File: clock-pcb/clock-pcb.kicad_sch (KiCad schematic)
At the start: 61 parts, among them J1 Conn_01x03_Pin, J10 Conn_01x01_Socket, J11 Conn_01x01_Socket, J12 Conn_01x01_Socket, J13 Conn_01x01_Socket, J14 Conn_01x01_Socket, J15 Conn_01x02_Socket, J2 oled, J3 Led display, J4 Led display 2, J5 Conn_01x07_Socket, J6 Conn_01x07_Socket, J7 Conn_01x01_Socket, J8 Conn_01x02_Socket, J9 Conn_01x01_Socket, Q1 FS8205A, Q2 FDN304PZ, U1 ESP32-WROOM-E, U4 TPS2116DRL, U5 MCP73811T-420I-OT, U7 TLV75533PDBV

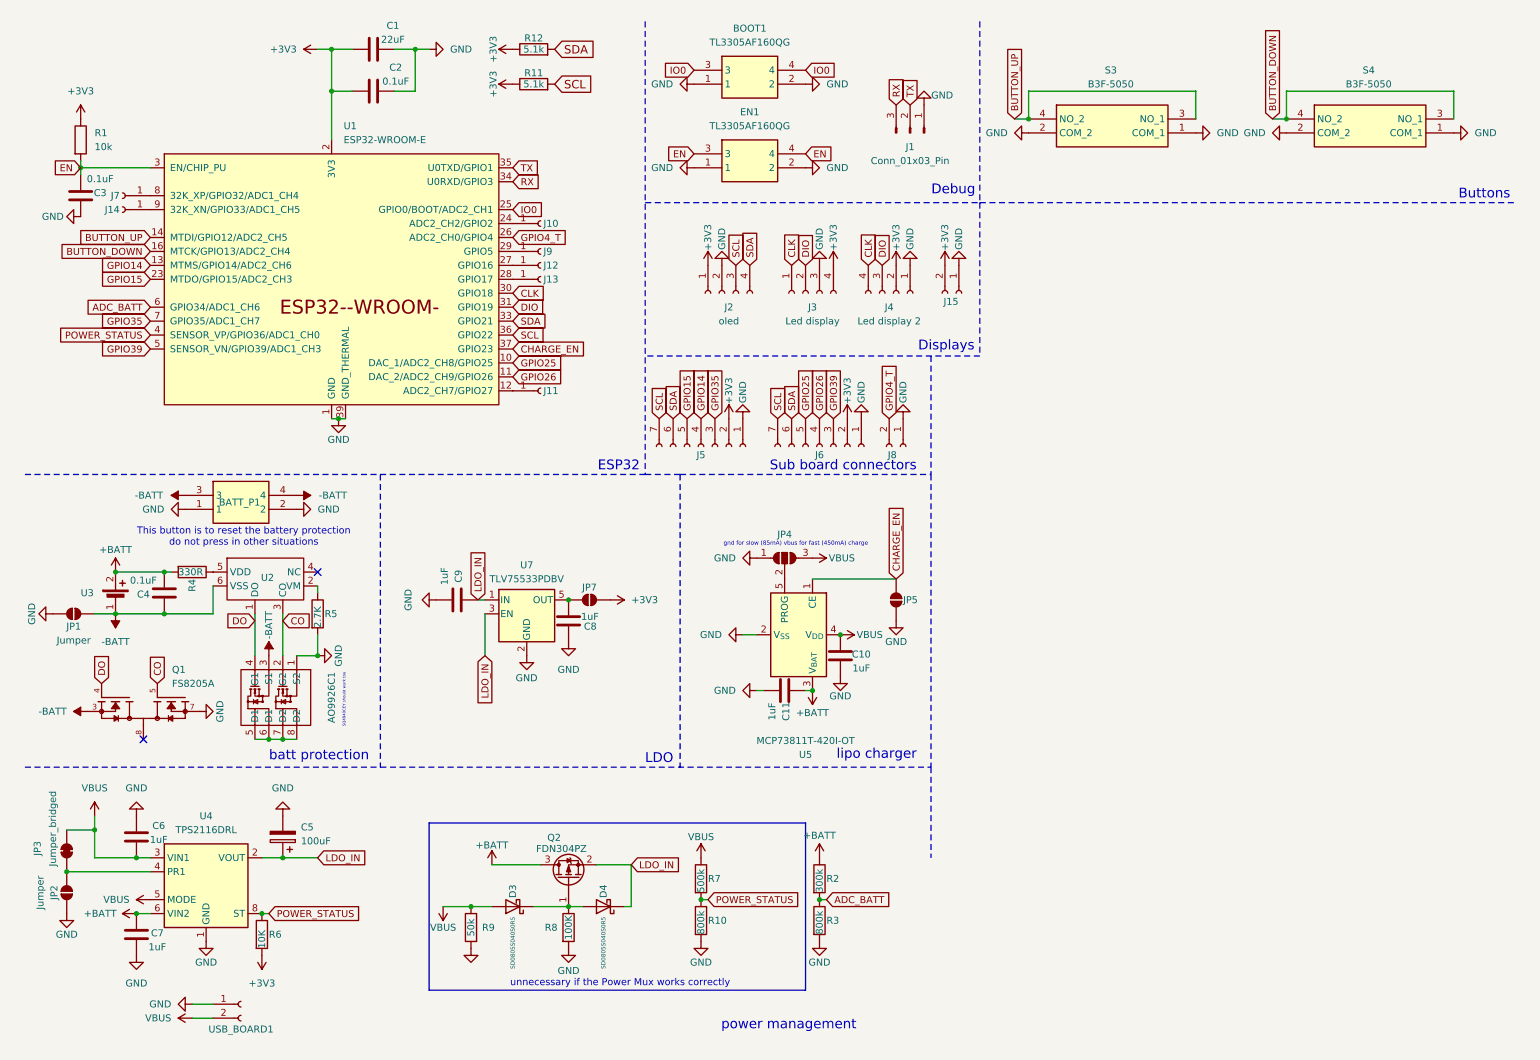
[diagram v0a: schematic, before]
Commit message: new pcb
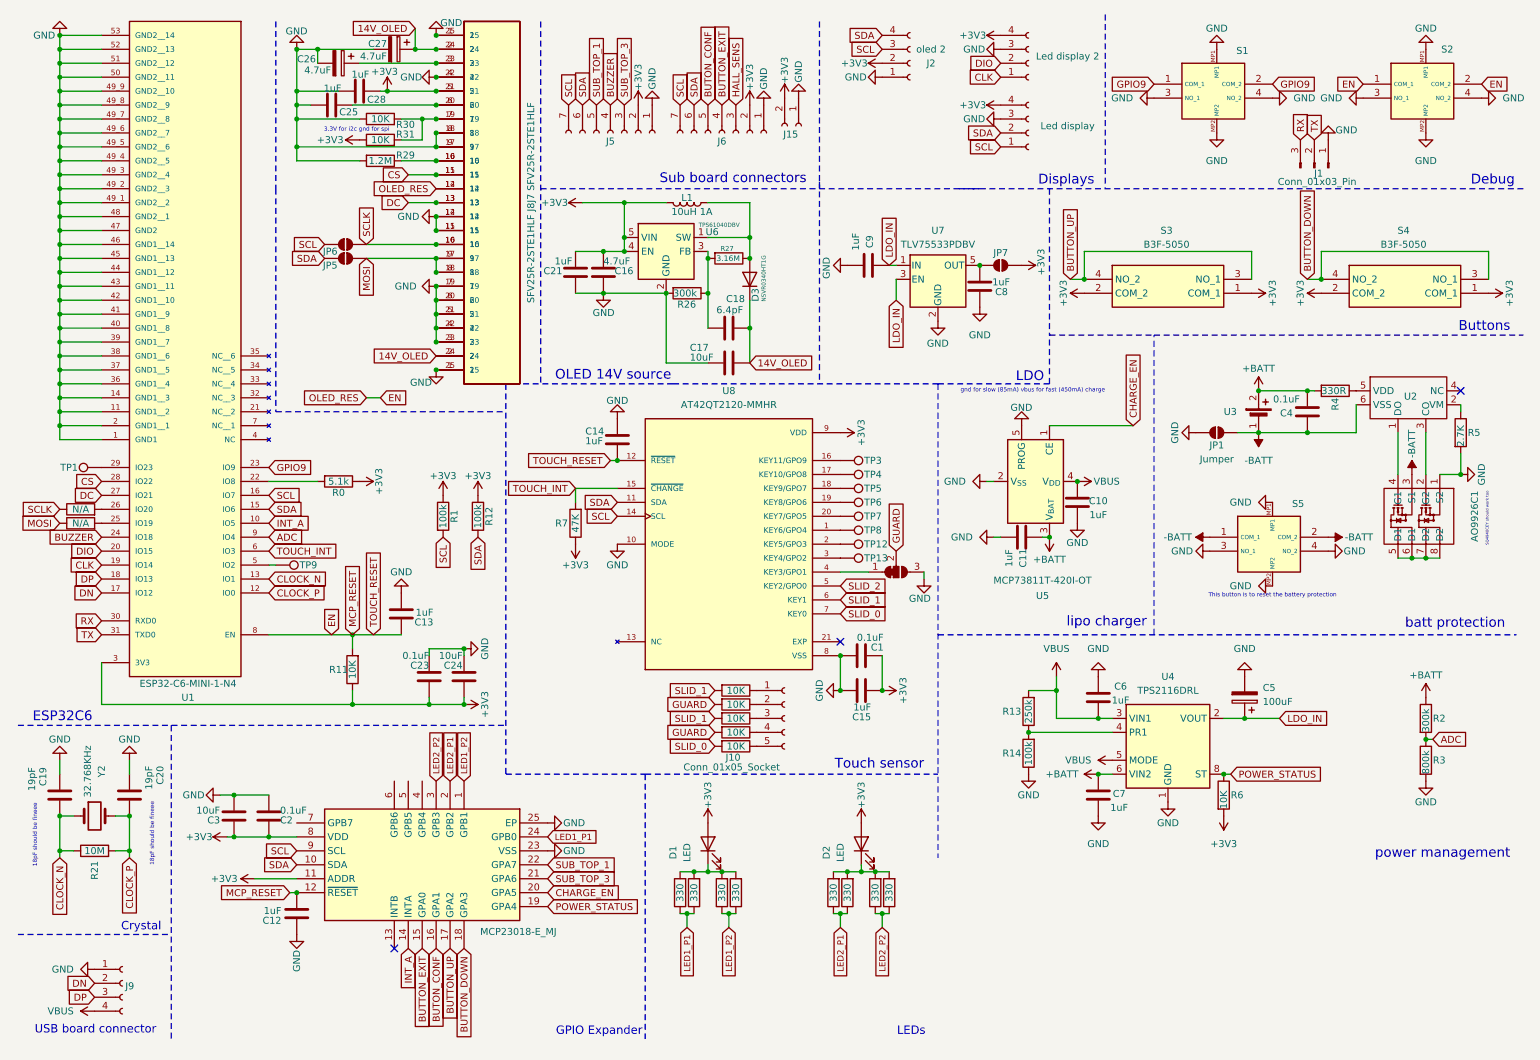
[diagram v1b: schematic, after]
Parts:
- removed BATT_P1, BOOT1, EN1: TL3305AF160QG, clock:TL3305AF160QG, symbol clock:TL3305AF160QG
- removed C1: 22uF, Capacitor_SMD:C_0805_2012Metric, symbol clock:C
- removed C2, C3: 0.1uF, Capacitor_SMD:C_0603_1608Metric, symbol clock:C
- removed D3, D4: SD0805S040S0R5, Diode_SMD:D_0805_2012Metric, symbol Watchy:D_Schottky
- removed J10, J11, J12, J13, J14, J7, J9: Conn_01x01_Socket, Connector_PinSocket_2.54mm:PinSocket_1x01_P2.54mm_Vertical, symbol Connector:Conn_01x01_Socket
- removed J5, J6: Conn_01x07_Socket, Connector_PinSocket_2.54mm:PinSocket_1x07_P2.54mm_Vertical, symbol Connector:Conn_01x07_Socket
- removed J8: Conn_01x02_Socket, Connector_PinSocket_2.54mm:PinSocket_1x02_P2.54mm_Vertical, symbol Connector:Conn_01x02_Socket
- removed JP2: Jumper, Jumper:SolderJumper-2_P1.3mm_Open_RoundedPad1.0x1.5mm, symbol Jumper:SolderJumper_2_Open
- removed JP3: Jumper_bridged, Jumper:SolderJumper-2_P1.3mm_Bridged2Bar_RoundedPad1.0x1.5mm, symbol Jumper:SolderJumper_2_Bridged
- removed JP4: SolderJumper_3_Open, Jumper:SolderJumper-3_P1.3mm_Open_RoundedPad1.0x1.5mm, symbol Jumper:SolderJumper_3_Open
- removed Q1: FS8205A, clock:SOP65P640X120-8N, symbol FS8205A:FS8205A
- removed Q2: FDN304PZ, Package_TO_SOT_SMD:SOT-23, symbol Watchy:BSS83P
- removed R1: 10k, Resistor_SMD:R_0402_1005Metric, symbol clock:R
- removed R10: 800k, Resistor_SMD:R_0402_1005Metric, symbol clock:R
- removed R7: 500k, Resistor_SMD:R_0402_1005Metric, symbol clock:R
- removed U1: ESP32-WROOM-E, PCM_Espressif:ESP32-WROOM-32E, symbol clock:ESP32-WROOM-E
- removed USB_BOARD1: Conn_01x02_Socket, clock:SHDR2W64P0X250_1X2_740X575X700P, symbol clock:Conn_01x02_Socket
- added C1, C2, C23: 0.1uF, Capacitor_SMD:C_0603_1608Metric, symbol Watchy:C
- added C12, C13, C14, C15, C21, C25, C28: 1uF, Capacitor_SMD:C_0603_1608Metric, symbol Watchy:C
- added C16: 4.7uF, Capacitor_SMD:C_0805_2012Metric, symbol Watchy:C
- added C17, C24, C3: 10uF, Capacitor_SMD:C_0603_1608Metric, symbol Watchy:C
- added C18: 6.4pF, Capacitor_SMD:C_0402_1005Metric, symbol Watchy:C
- added C19, C20: 19pF, Capacitor_SMD:C_0402_1005Metric, symbol Watchy:C
- added C26, C27: 4.7uF, Capacitor_Tantalum_SMD:CP_EIA-3528-12_Kemet-T, symbol Device:C_Polarized
- added D1, D2: LED, LED_SMD:LED_1210_3225Metric, symbol Device:LED
- added D3: NSVR0340HT1G, Diode_SMD:D_SOD-323, symbol Device:D
- added IC2: MCP23018-E_MJ, clock:QFN50P400X400X90-25N-D, symbol Watchy:MCP23018-E_MJ
- added J10: Conn_01x05_Socket, Connector_PinHeader_2.54mm:PinHeader_1x05_P2.54mm_Vertical, symbol Connector:Conn_01x05_Socket
- added J5, J6: Conn_01x07_Socket, Connector_PinHeader_2.54mm:PinHeader_1x07_P2.54mm_Vertical, symbol clock:Conn_01x07_Socket
- added J7: SFV25R-2STE1HLF, clock:OLED_1.5IN_128X128MONO, symbol SFV25R-2STE1HLF:SFV25R-2STE1HLF
- added J8: SFV25R-2STE1HLF, clock:AMPHENOL_SFV25R-2STE1HLF, symbol SFV25R-2STE1HLF:SFV25R-2STE1HLF
- added J9: Conn_01x04_Socket, Connector_JST:JST_XH_B4B-XH-AM_1x04_P2.50mm_Vertical, symbol Connector:Conn_01x04_Socket
- added JP2: SolderJumper_3_Bridged12, clock:jumper_solder_small_3_bridged, symbol Jumper:SolderJumper_3_Bridged12
- added JP6: Jumper, clock:jumper_solder_small, symbol Jumper:SolderJumper_2_Open
- added L1: 10uH 1A, clock:HPI0530-100, symbol Watchy:L
- added R0: 5.1k, Resistor_SMD:R_0402_1005Metric, symbol Watchy:R
- added R1, R14: 100k, Resistor_SMD:R_0402_1005Metric, symbol Watchy:R
- added R10, R15, R16, R30, R31: 10K, Resistor_SMD:R_0402_1005Metric, symbol Watchy:R
- added R13: 250k, Resistor_SMD:R_0402_1005Metric, symbol Watchy:R
- added R17, R18, R19, R20, R22, R23, R24, R25: 330, Resistor_SMD:R_0402_1005Metric, symbol Yatchy:R
- added R21: 10M, Resistor_SMD:R_0402_1005Metric, symbol Watchy:R
- added R26: 300k, Resistor_SMD:R_0402_1005Metric, symbol Watchy:R
- added R27: 3.16M, Resistor_SMD:R_0402_1005Metric, symbol Watchy:R
- added R29: 1.2M, Resistor_SMD:R_0402_1005Metric, symbol Watchy:R
- added R32, R33: N/A, Resistor_SMD:R_0402_1005Metric, symbol Watchy:R
- added R7: 47K, Resistor_SMD:R_0402_1005Metric, symbol Watchy:R
- added S1, S2, S5: TS21-34-035-BK-160-SMT-TR, TS2134035BK160SMTTR, symbol TS21-34-035-BK-160-SMT-TR:TS21-34-035-BK-160-SMT-TR
- added TP1, TP12, TP13, TP3, TP4, TP5, TP6, TP7, TP8, TP9: TestPoint, TestPoint:TestPoint_THTPad_1.0x1.0mm_Drill0.5mm, symbol Connector:TestPoint
- added U1: ESP32-C6-MINI-1-N4, clock:XCVR_ESP32-C6-MINI-1-N4, symbol Watchy:ESP32-C6-MINI-1-N4
- added U6: TPS61040DBV, Package_TO_SOT_SMD:SOT-23-5, symbol Regulator_Switching:TPS61040DBV
- added U8: AT42QT2120-MMHR, clock:QFN45P300X300X85-21N, symbol AT42QT2120-MMHR:AT42QT2120-MMHR
- added Y2: 32.768KHz, clock:XTAL_9HT10_TXC, symbol Watchy:Crystal
- J2: value oled -> oled 2
- JP1, JP7: footprint Jumper:SolderJumper-2_P1.3mm_Open_RoundedPad1.0x1.5mm -> clock:jumper_solder_small
- JP5: value SolderJumper_2_Open -> Jumper; footprint Jumper:SolderJumper-2_P1.3mm_Open_RoundedPad1.0x1.5mm -> clock:jumper_solder_small
- R11: value 5.1k -> 10K
- R12: value 5.1k -> 100k
- R8: value 100K -> 10K
- R9: value 50k -> 10K
- U3: footprint clock:SHDR2W64P0X250_1X2_740X575X700P -> Connector_JST:JST_XH_B2B-XH-AM_1x02_P2.50mm_Vertical
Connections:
- net +3V3: now also J2.2 (Pin_2), J4.4 (Pin_4), S3.1 (COM_1), S3.2 (COM_2), S4.1 (COM_1), S4.2 (COM_2), C1.2, C15.2, C16.1, C2.1, C21.2, C23.1, C24.1, C28.2, C3.1, D1.2 (A), D2.2 (A), IC2.11 (ADDR), IC2.8 (VDD), J5.2 (Pin_2), J6.2 (Pin_2), J7.5, J8.21, L1.2, R0.1, R1.1, R31.1, R7.1, U1.3 (3V3), U6.4 (EN), U6.5 (VIN), U8.9 (VDD); no longer J2.1 (Pin_1), J4.2 (Pin_2)
- net -BATT: now also S5.1 (COM_1), S5.2 (COM_2)
- net BUTTON_DOWN: now also IC2.18 (GPA3)
- net BUTTON_UP: now also IC2.17 (GPA2)
- net CHARGE_EN: now also IC2.20 (GPA5); no longer JP5.2 (B)
- net CLK: now also J4.1 (Pin_1), U1.19 (IO14); no longer J3.1 (Pin_1), J4.4 (Pin_4)
- net DIO: now also J4.2 (Pin_2), U1.20 (IO15); no longer J3.2 (Pin_2), J4.3 (Pin_3)
- net EN: now also R11.2, C12.2, C13.1, C14.2, IC2.12 (~{RESET}), J7.12, J8.14, S2.1 (COM_1), S2.2 (COM_2), U1.8 (EN), U8.12 (~{RESET})
- net GND: now also J2.1 (Pin_1), J4.3 (Pin_3), U5.5 (PROG), C1.1, C12.1, C13.2, C14.1, C15.1, C16.2, C17.2, C19.2, C2.2, C20.2, C21.1, C23.2, C24.2, C25.1, C26.2, C27.2, C28.1, C3.2, IC2.23 (VSS), IC2.25 (EP), J5.1 (Pin_1), J6.1 (Pin_1), J7.1, J7.14, J7.15, J7.19, J7.20, J7.21, J7.22, J7.23, J7.25, J7.4, J7.8, J7.9, J8.1, J8.11, J8.12, J8.17, J8.18, J8.22, J8.25, J8.3, J8.4, J8.5, J8.6, J8.7, J9.1 (Pin_1), JP2.3 (B), R14.1, R26.2, R29.2, R30.1, S1.3 (NO_1), S1.4 (NO_2), S1.MP1, S1.MP2, S2.3 (NO_1), S2.4 (NO_2), S2.MP1, S2.MP2, S5.3 (NO_1), S5.4 (NO_2), S5.MP1, S5.MP2, U1.1 (GND1), U1.11 (GND1__2), U1.14 (GND1__3), U1.2 (GND1__1), U1.36 (GND1__4), U1.37 (GND1__5), U1.38 (GND1__6), U1.39 (GND1__7), U1.40 (GND1__8), U1.41 (GND1__9), U1.42 (GND1__10), U1.43 (GND1__11), U1.44 (GND1__12), U1.45 (GND1__13), U1.46 (GND1__14), U1.47 (GND2), U1.48 (GND2__1), U1.49_1 (GND2__2), U1.49_2 (GND2__3), U1.49_3 (GND2__4), U1.49_4 (GND2__5), U1.49_5 (GND2__6), U1.49_6 (GND2__7), U1.49_7 (GND2__8), U1.49_8 (GND2__9), U1.49_9 (GND2__10), U1.50 (GND2__11), U1.51 (GND2__12), U1.52 (GND2__13), U1.53 (GND2__14), U6.2 (GND), U8.10 (MODE), U8.8 (VSS); no longer J2.2 (Pin_2), J4.1 (Pin_1), JP5.1 (A), R8.2, R9.2, S3.1 (COM_1), S3.2 (COM_2), S4.1 (COM_1), S4.2 (COM_2)
- net POWER_STATUS: now also IC2.19 (GPA4)
- net RX: now also U1.30 (RXD0)
- net SCL: now also J3.1 (Pin_1), IC2.9 (SCL), J5.7 (Pin_7), J6.7 (Pin_7), JP6.1 (A), R1.2, U1.16 (IO7), U8.14 (SCL); no longer R11.2
- net SDA: now also J3.2 (Pin_2), JP5.1 (A), IC2.10 (SDA), J5.6 (Pin_6), J6.6 (Pin_6), U1.15 (IO6), U8.11 (SDA)
- net TX: now also U1.31 (TXD0)
- net VBUS: now also J9.4 (Pin_4), R13.2; no longer R9.1
- net at R8.1: now also J10.5 (Pin_5)
- net at U4.4 (PR1): now also R13.1, R14.2
- net ADC_BATT renamed ADC
- net ADC: now also U1.9 (IO4)
- net CO: no longer names the net of AO9926C1.2 (G2), U2.3 (CO)
- net DO: no longer names the net of AO9926C1.4 (G1), U2.1 (DO)
- new net: D3.2 (A), L1.1, R27.1, U6.1 (SW)
- new net: C18.2, R26.1, R27.2, U6.3 (FB)
- new net: D2.1 (K), R22.2, R23.2, R24.2, R25.2
- new net: J10.2 (Pin_2), R15.1
- new net: TP3.1, U8.16 (KEY11/GPO9)
- new net: D1.1 (K), R17.2, R18.2, R19.2, R20.2
- new net: C26.1, J7.3, J8.23
- new net: TP8.1, U8.1 (KEY6/GPO4)
- new net: TP4.1, U8.17 (KEY10/GPO8)
- new net: TP5.1, U8.18 (KEY9/GPO7)
- new net: TP6.1, U8.19 (KEY8/GPO6)
- new net: TP12.1, U8.2 (KEY5/GPO3)
- new net: TP7.1, U8.20 (KEY7/GPO5)
- new net: TP13.1, U8.3 (KEY4/GPO2)
- new net: JP2.1 (A), U8.4 (KEY3/GPO1)
- new net: J10.4 (Pin_4), R9.1
- new net: R0.2, U1.22 (IO8)
- new net: TP1.1, U1.29 (IO23)
- new net: J10.3 (Pin_3), R10.1
- new net: TP9.1, U1.5 (IO2)
- new net: J7.10, J8.16, R29.1
- new net: C25.2, J7.6, J8.20
- new net: J7.7, J8.19, R30.2, R31.2
- new net: J10.1 (Pin_1), R16.1
- new net: R33.2, U1.25 (IO19)
- new net: R32.2, U1.26 (IO20)
- new net 14V_OLED: C17.1, C18.1, C27.1, D3.1 (K), J7.2, J7.24, J8.2, J8.24
- new net BUTON_CONF: IC2.16 (GPA1), J6.5 (Pin_5)
- new net BUTTON_EXIT: IC2.15 (GPA0), J6.4 (Pin_4)
- new net BUZZER: J5.4 (Pin_4), U1.24 (IO18)
- new net CLOCK_N: C19.1, R21.1, U1.13 (IO1), Y2.1
- new net CLOCK_P: C20.1, R21.2, U1.12 (IO0), Y2.2
- new net CS: J7.11, J8.15, U1.28 (IO22)
- new net DC: J7.13, J8.13, U1.27 (IO21)
- new net DN: J9.2 (Pin_2), U1.17 (IO12)
- new net DP: J9.3 (Pin_3), U1.18 (IO13)
- new net GPIO9: S1.1 (COM_1), S1.2 (COM_2), U1.23 (IO9)
- new net GUARD: JP2.2 (C), R15.2, R9.2
- new net HALL_SENS: J6.3 (Pin_3)
- new net INT_A: IC2.14 (INTA), U1.10 (IO5)
- new net LED1_P1: IC2.24 (GPB0), R17.1, R19.1
- new net LED1_P2: IC2.1 (GPB1), R18.1, R20.1
- new net LED2_P1: IC2.2 (GPB2), R22.1, R23.1
- new net LED2_P2: IC2.3 (GPB3), R24.1, R25.1
- new net MOSI: J7.17, J7.18, J8.8, J8.9, JP5.2 (B), R33.1
- new net SCLK: J7.16, J8.10, JP6.2 (B), R32.1
- new net SLID_0: R8.2, U8.7 (KEY0)
- new net SLID_1: R10.2, R16.2, U8.6 (KEY1)
- new net SLID_2: U8.5 (KEY2/GPO0)
- new net SUB_TOP_1: IC2.22 (GPA7), J5.5 (Pin_5)
- new net SUB_TOP_3: IC2.21 (GPA6), J5.3 (Pin_3)
- new net TOUCH_INT: R7.2, U1.6 (IO3), U8.15 (~{CHANGE})
- no-connect marks 2 -> 3
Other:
- note added: "18pF should be fineee"
- note added: "3.3V for i2c gnd for spi"
- note added: "Crystal"
- note added: "ESP32C6"
- note added: "GPIO Expander"
- note added: "LEDs"
- note added: "OLED 14V source"
- note added: "This button is to reset the battery protection"
- note added: "Touch sensor"
- note added: "USB board connector"
- note removed: "ESP32"
- note removed: "This button is to reset the battery protection do not press in other situations"
- note removed: "unnecessary if the Power Mux works correctly"
- moved on the sheet: AO9926C1, C10, C11, C4, C5, C6, C7, C8, C9, J1, J15, J2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

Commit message: routing
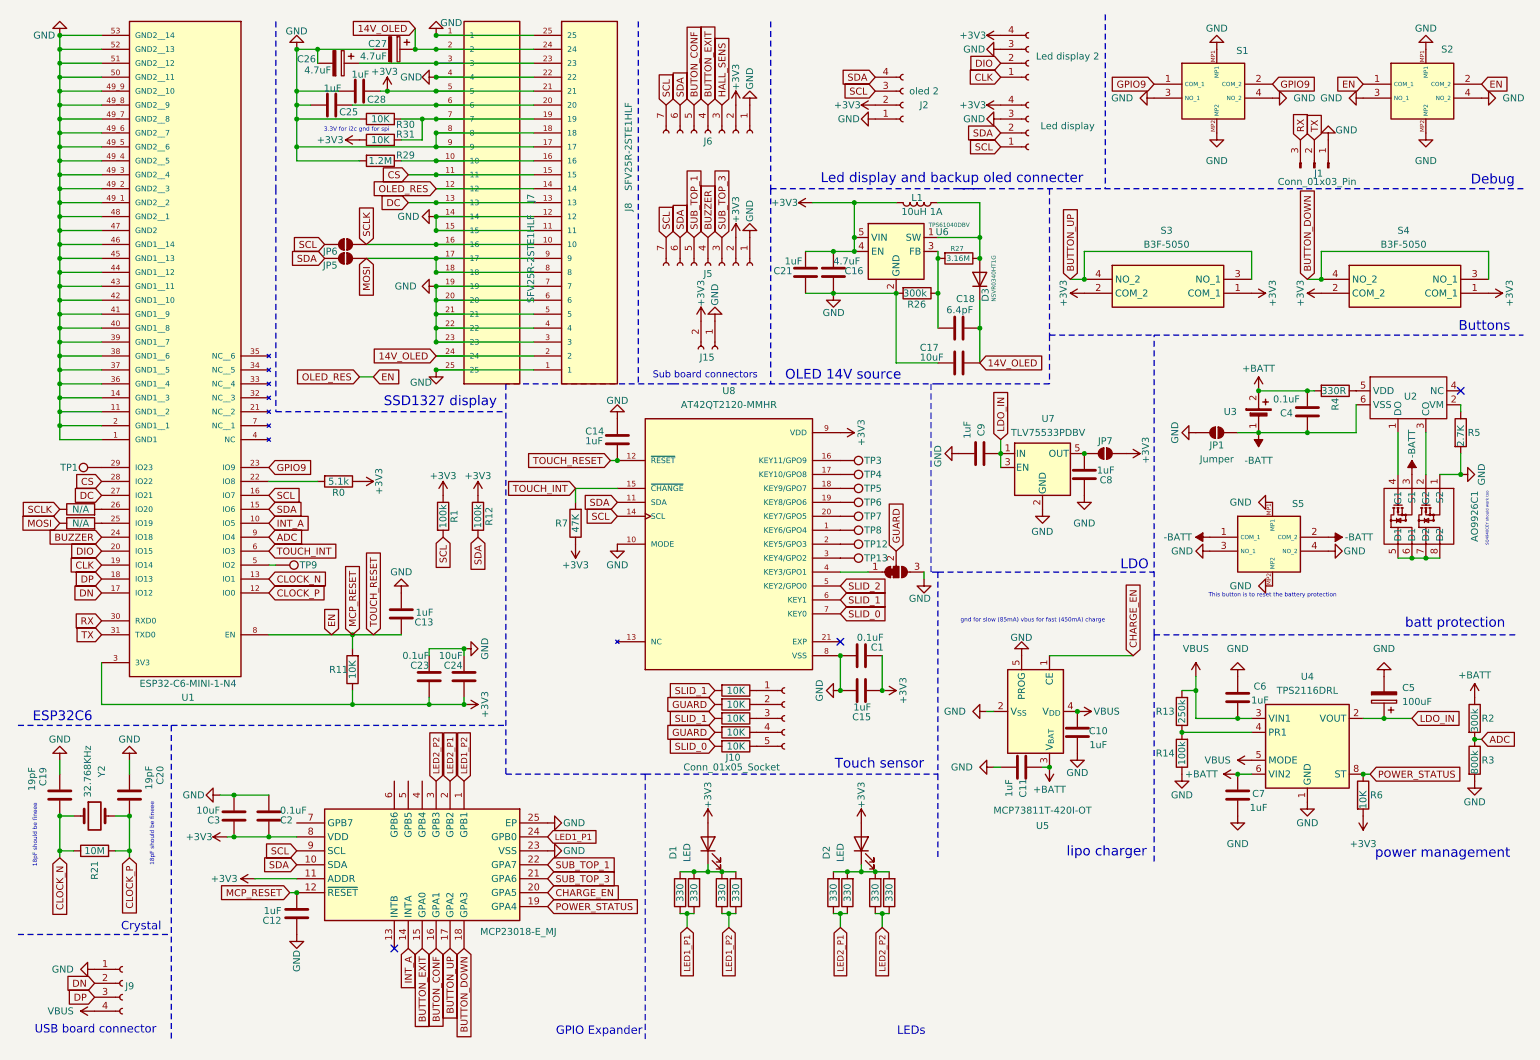
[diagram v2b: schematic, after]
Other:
- note added: "Led display and backup oled connecter"
- note added: "SSD1327 display"
- note removed: "Displays"
- moved on the sheet: C10, C11, C16, C17, C18, C21, C5, C6, C7, C8, C9, D3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
